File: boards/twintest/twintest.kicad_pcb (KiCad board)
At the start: 4 copper layers, 38.1 x 57.2 mm, 26 parts, among them J1 USB_C, SW1 SW_Push, U1 STM32F072CBT6, U3 XC6206, U4 USBLC6-2SC6

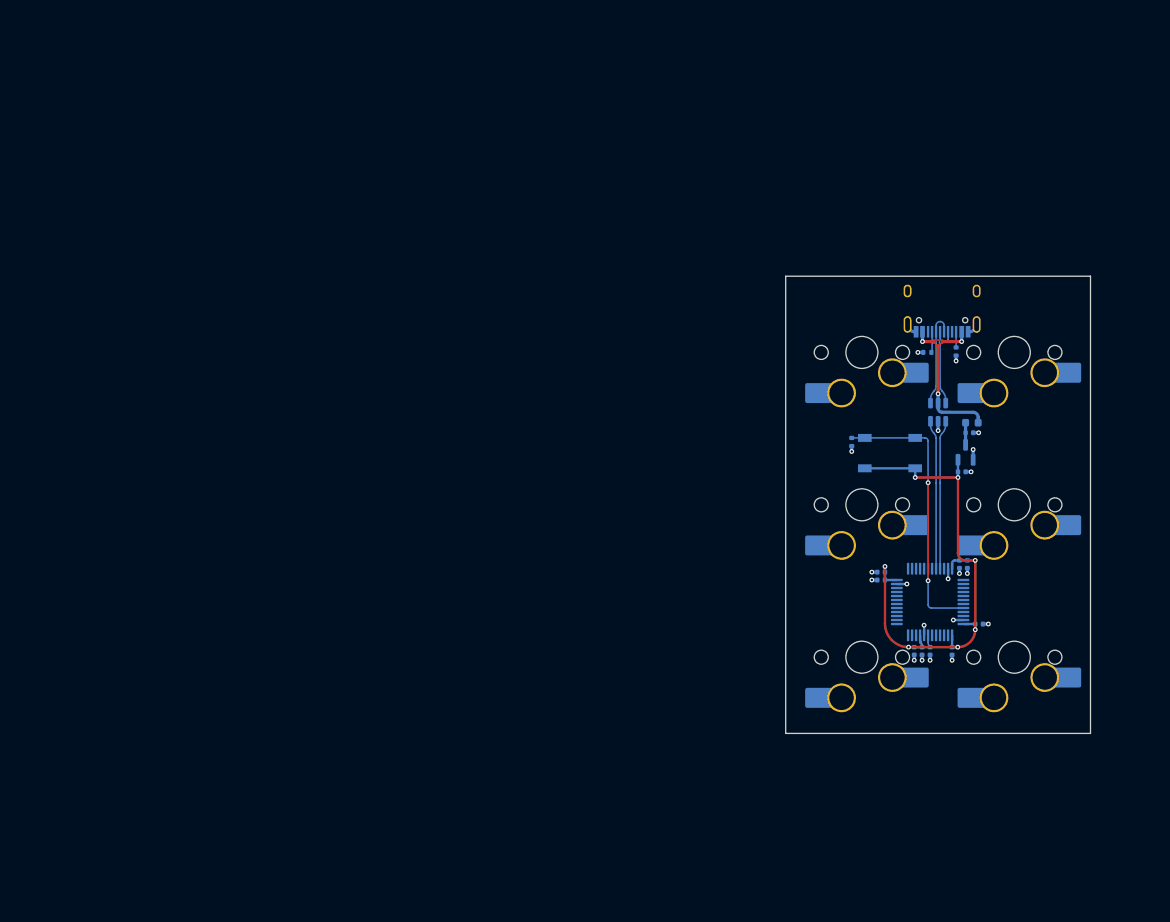
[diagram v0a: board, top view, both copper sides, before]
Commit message: update
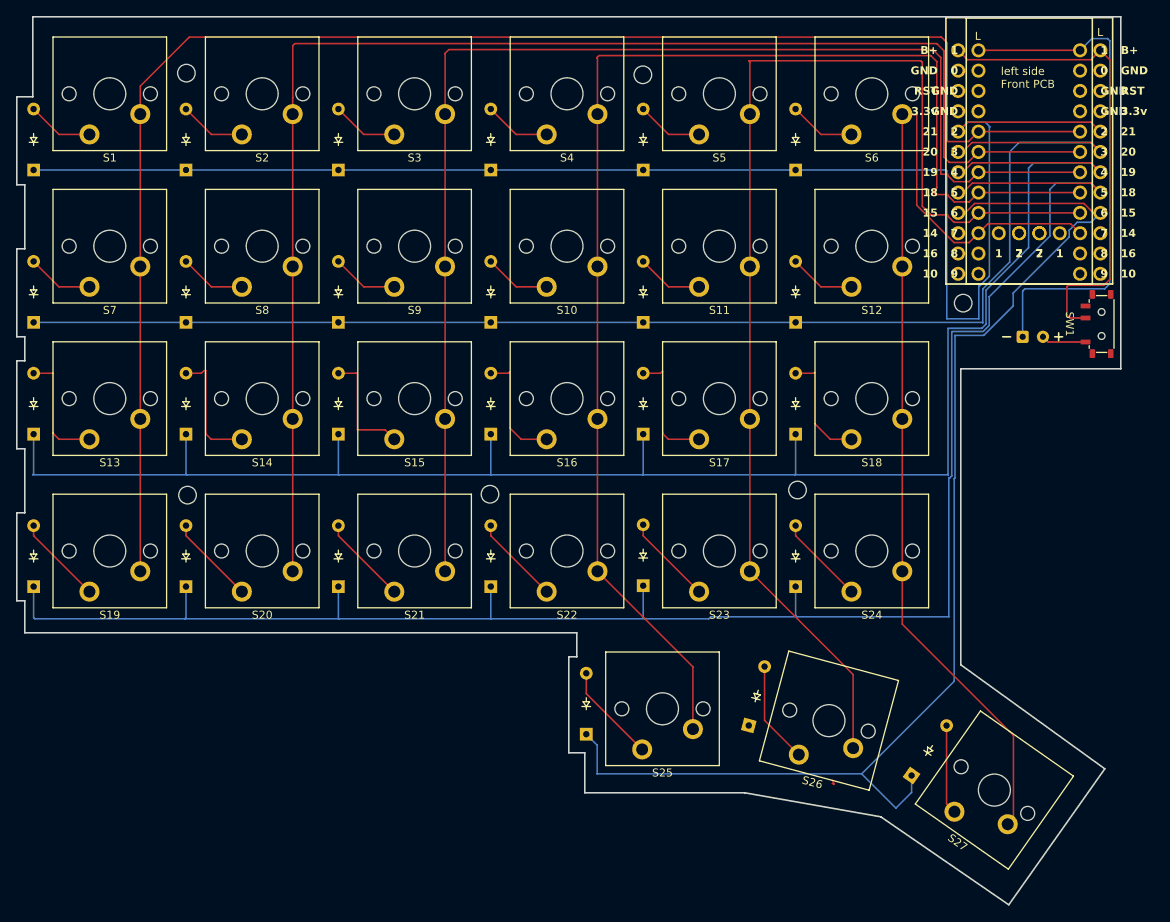
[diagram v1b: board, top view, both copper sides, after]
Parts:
- removed C10, C11, C13, C16, C7: 100nF, ScottoKeebs_Components:Capacitor_0402
- removed C12, C17: 4.7uF, ScottoKeebs_Components:Capacitor_0402
- removed C14: 10nF, ScottoKeebs_Components:Capacitor_0402
- removed C15, C8, C9: 1uF, ScottoKeebs_Components:Capacitor_0402
- removed F1: 500mA, ScottoKeebs_Components:Fuse_0603
- removed J1: USB_C, ScottoKeebs_Components:USB_C_HRO_TYPE-C-31-M-12
- removed R1: 10k, ScottoKeebs_Components:Resistor_0402
- removed R2, R3: 5.1k, ScottoKeebs_Components:Resistor_0402
- removed REF** (x6): MX_1.00u_PG151101S11, ScottoKeebs_Scotto:MX_Hotswap_1.00u
- removed U3: XC6206, ScottoKeebs_Components:Voltage_SOT-23
- removed U4: USBLC6-2SC6, ScottoKeebs_Components:ESD_SOT-23-6
- added BT2: Battery_Cell, ScottoKeebs_Scotto:Battery, F.Cu at (163.0, 78.0)
- added D1: Diode, ScottoKeebs_Components:Diode_DO-35, F.Cu at (38.1, 57.1)
- added D10: Diode, ScottoKeebs_Components:Diode_DO-35, F.Cu at (95.2, 76.2)
- added D11: Diode, ScottoKeebs_Components:Diode_DO-35, F.Cu at (114.3, 76.2)
- added D12: Diode, ScottoKeebs_Components:Diode_DO-35, F.Cu at (133.3, 76.2)
- added D13: Diode, ScottoKeebs_Components:Diode_DO-35, F.Cu at (38.1, 90.2)
- added D14: Diode, ScottoKeebs_Components:Diode_DO-35, F.Cu at (57.1, 90.2)
- added D15: Diode, ScottoKeebs_Components:Diode_DO-35, F.Cu at (76.2, 90.2)
- added D16: Diode, ScottoKeebs_Components:Diode_DO-35, F.Cu at (95.2, 90.2)
- added D17: Diode, ScottoKeebs_Components:Diode_DO-35, F.Cu at (114.3, 90.2)
- added D18: Diode, ScottoKeebs_Components:Diode_DO-35, F.Cu at (133.3, 90.2)
- added D19: Diode, ScottoKeebs_Components:Diode_DO-35, F.Cu at (38.1, 109.2)
- added D2: Diode, ScottoKeebs_Components:Diode_DO-35, F.Cu at (57.1, 57.1)
- added D20: Diode, ScottoKeebs_Components:Diode_DO-35, F.Cu at (57.1, 109.2)
- added D21: Diode, ScottoKeebs_Components:Diode_DO-35, F.Cu at (76.2, 109.2)
- added D22: Diode, ScottoKeebs_Components:Diode_DO-35, F.Cu at (95.2, 109.2)
- added D23: Diode, ScottoKeebs_Components:Diode_DO-35, F.Cu at (114.3, 109.1)
- added D24: Diode, ScottoKeebs_Components:Diode_DO-35, F.Cu at (133.3, 109.2)
- added D25: Diode, ScottoKeebs_Components:Diode_DO-35, F.Cu at (107.2, 127.7)
- added D26: Diode, ScottoKeebs_Components:Diode_DO-35, F.Cu at (127.5, 126.6)
- added D27: Diode, ScottoKeebs_Components:Diode_DO-35, F.Cu at (147.8, 132.8)
- added D3: Diode, ScottoKeebs_Components:Diode_DO-35, F.Cu at (76.2, 57.1)
- added D4: Diode, ScottoKeebs_Components:Diode_DO-35, F.Cu at (95.2, 57.1)
- added D5: Diode, ScottoKeebs_Components:Diode_DO-35, F.Cu at (114.3, 57.1)
- added D6: Diode, ScottoKeebs_Components:Diode_DO-35, F.Cu at (133.3, 57.1)
- added D7: Diode, ScottoKeebs_Components:Diode_DO-35, F.Cu at (38.1, 76.2)
- added D8: Diode, ScottoKeebs_Components:Diode_DO-35, F.Cu at (57.1, 76.2)
- added D9: Diode, ScottoKeebs_Components:Diode_DO-35, F.Cu at (76.2, 76.2)
- added H1: Mounting_Hole, ScottoKeebs_Scotto:Standoff_M2x6mm, F.Cu at (57.2, 45.0)
- added H2: Mounting_Hole, ScottoKeebs_Scotto:Standoff_M2x6mm, F.Cu at (57.3, 97.8)
- added H3: Mounting_Hole, ScottoKeebs_Scotto:Standoff_M2x6mm, F.Cu at (114.3, 45.2)
- added H4: Mounting_Hole, ScottoKeebs_Scotto:Standoff_M2x6mm, F.Cu at (95.2, 97.7)
- added H5: Mounting_Hole, ScottoKeebs_Scotto:Standoff_M2x6mm, F.Cu at (154.3, 73.8)
- added H6: Mounting_Hole, ScottoKeebs_Scotto:Standoff_M2x6mm, F.Cu at (133.6, 97.2)
- added S1: Keyswitch, ScottoKeebs_MX:MX_PCB_1.00u, F.Cu at (47.6, 47.6)
- added S10: Keyswitch, ScottoKeebs_MX:MX_PCB_1.00u, F.Cu at (104.8, 66.7)
- added S11: Keyswitch, ScottoKeebs_MX:MX_PCB_1.00u, F.Cu at (123.8, 66.7)
- added S12: Keyswitch, ScottoKeebs_MX:MX_PCB_1.00u, F.Cu at (142.9, 66.7)
- added S13: Keyswitch, ScottoKeebs_MX:MX_PCB_1.00u, F.Cu at (47.6, 85.7)
- added S14: Keyswitch, ScottoKeebs_MX:MX_PCB_1.00u, F.Cu at (66.7, 85.7)
- added S15: Keyswitch, ScottoKeebs_MX:MX_PCB_1.00u, F.Cu at (85.7, 85.7)
- added S16: Keyswitch, ScottoKeebs_MX:MX_PCB_1.00u, F.Cu at (104.8, 85.7)
- added S17: Keyswitch, ScottoKeebs_MX:MX_PCB_1.00u, F.Cu at (123.8, 85.7)
- added S18: Keyswitch, ScottoKeebs_MX:MX_PCB_1.00u, F.Cu at (142.9, 85.7)
- added S19: Keyswitch, ScottoKeebs_MX:MX_PCB_1.00u, F.Cu at (47.6, 104.8)
- added S2: Keyswitch, ScottoKeebs_MX:MX_PCB_1.00u, F.Cu at (66.7, 47.6)
- added S20: Keyswitch, ScottoKeebs_MX:MX_PCB_1.00u, F.Cu at (66.7, 104.8)
- added S21: Keyswitch, ScottoKeebs_MX:MX_PCB_1.00u, F.Cu at (85.7, 104.8)
- added S22: Keyswitch, ScottoKeebs_MX:MX_PCB_1.00u, F.Cu at (104.8, 104.8)
- added S23: Keyswitch, ScottoKeebs_MX:MX_PCB_1.00u, F.Cu at (123.8, 104.8)
- added S24: Keyswitch, ScottoKeebs_MX:MX_PCB_1.00u, F.Cu at (142.9, 104.8)
- added S25: Keyswitch, ScottoKeebs_MX:MX_PCB_1.00u, F.Cu at (116.7, 124.5)
- added S26: Keyswitch, ScottoKeebs_MX:MX_PCB_1.00u, F.Cu at (137.5, 126.0)
- added S27: Keyswitch, ScottoKeebs_MX:MX_PCB_1.00u, F.Cu at (158.2, 134.7)
- added S3: Keyswitch, ScottoKeebs_MX:MX_PCB_1.00u, F.Cu at (85.7, 47.6)
- added S4: Keyswitch, ScottoKeebs_MX:MX_PCB_1.00u, F.Cu at (104.8, 47.6)
- added S5: Keyswitch, ScottoKeebs_MX:MX_PCB_1.00u, F.Cu at (123.8, 47.6)
- added S6: Keyswitch, ScottoKeebs_MX:MX_PCB_1.00u, F.Cu at (142.9, 47.6)
- added S7: Keyswitch, ScottoKeebs_MX:MX_PCB_1.00u, F.Cu at (47.6, 66.7)
- added S8: Keyswitch, ScottoKeebs_MX:MX_PCB_1.00u, F.Cu at (66.7, 66.7)
- added S9: Keyswitch, ScottoKeebs_MX:MX_PCB_1.00u, F.Cu at (85.7, 66.7)
- added U2: Nice_Nano_V2, ScottoKeebs_MCU:Nice_Nano_V2, B.Cu at (161.3, 55.9)
- SW1: value SW_Push -> Switch; footprint ScottoKeebs_Components:Button_TL3342 -> ScottoKeebs_Components:Switch_MSK12C02; moved to F.Cu
- U1: value STM32F072CBT6 -> Nice_Nano_V2; footprint ScottoKeebs_Components:Package_LQFP-48_7x7mm_P0.5 -> ScottoKeebs_MCU:Nice_Nano_V2; moved to F.Cu
- moved U1 56.9 mm to (163.8, 55.9), turned to 0 degrees
- moved SW1 31.0 mm to (171.6, 76.4), turned to -90 degrees
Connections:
- SW1 pad 1: +3.3V -> Net-(BT2-+)
- SW1 pad 2: /BOOT0 -> battery +
- U1 pad 1: +3.3V -> battery -
- U1 pad 10: /A0 -> collumn 6
- U1 pad 11: /A1 -> unconnected-(U1-8-Pad11)
- U1 pad 12: /A2 -> unconnected-(U1-9-Pad12)
- U1 pad 13: /A3 -> unconnected-(U1-10-Pad13)
- U1 pad 14: /A4 -> unconnected-(U1-16-Pad14)
- U1 pad 15: /A5 -> unconnected-(U1-14-Pad15)
- U1 pad 16: /A6 -> row 5
- U1 pad 17: /A7 -> row 4
- U1 pad 18: /B0 -> row 3
- U1 pad 19: /B1 -> row 2
- U1 pad 2: /C13 -> unconnected-(U1-0-Pad2)
- U1 pad 20: /B2 -> row 1
- U1 pad 21: /B10 -> unconnected-(U1-3.3v-Pad21)
- U1 pad 22: /B11 -> unconnected-(U1-RST-Pad22)
- U1 pad 23: GND -> unconnected-(U1-GND-Pad23)
- U1 pad 24: +3.3V -> battery +
- U1 pad 25: /B12 -> unconnected-(U1-1-Pad25)
- U1 pad 26: /B13 -> unconnected-(U1-2-Pad26)
- U1 pad 27: /B14 -> unconnected-(U1-7-Pad27)
- U1 pad 3: /C14 -> unconnected-(U1-GND-Pad3)
- U1 pad 4: /C15 -> unconnected-(U1-GND-Pad4)
- U1 pad 5: /F0 -> collumn 1
- U1 pad 6: /F1 -> collumn 2
- U1 pad 7: /NRST -> collumn 3
- U1 pad 8: GND -> collumn 4
- U1 pad 9: +3.3V -> collumn 5
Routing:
- net row 4: track 0.00 -> 225.5 mm
- net row 3: track 0.00 -> 218.6 mm
- net collumn 1: track 0.00 -> 194.5 mm
- net row 1: track 0.00 -> 184.9 mm
- net collumn 2: track 0.00 -> 178.7 mm
- net row 2: track 0.00 -> 172.7 mm
- net collumn 4: track 0.00 -> 167.9 mm
- net collumn 3: track 0.00 -> 160.4 mm
- net row 5: track 0.00 -> 153.9 mm
- net collumn 5: track 0.00 -> 152.3 mm
- net collumn 6: track 0.00 -> 131.8 mm
- net +3.3V: track 71.5 -> 0.00 mm, vias 7 -> 0
- net battery -: track 0.00 -> 64.5 mm
- net battery +: track 0.00 -> 59.7 mm
- net /BOOT0: track 34.8 -> 0.00 mm, vias 2 -> 0
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- removed copper zone on B.Cu, net /USB_D+
- removed copper zone on In1.Cu, net GND
- removed copper zone on In2.Cu, net GND
- removed copper zone on F.Cu, net VBUS
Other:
- board size 38.1 x 57.2 mm -> 138 x 111 mm
- copper layers 4 -> 2
- board text added: "L"
- board text added: "R"
- board text added: "left side Front PCB"
- board text removed: "JLCJLCJLCJLC"
